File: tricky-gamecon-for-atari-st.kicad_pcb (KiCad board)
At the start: 2 copper layers, 14 parts, among them J1 Conn_01x09, SW1 GrayHill_series_78_SPDT_DIP_x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, SW2 SW_SPST, SW3 SW_SPST, SW4 SW_SPST, SW5 SW_SPST, SW6 SW_SPST, SW7 SW_SPST, SW8 SW_SPST, SW9 SW_SPST

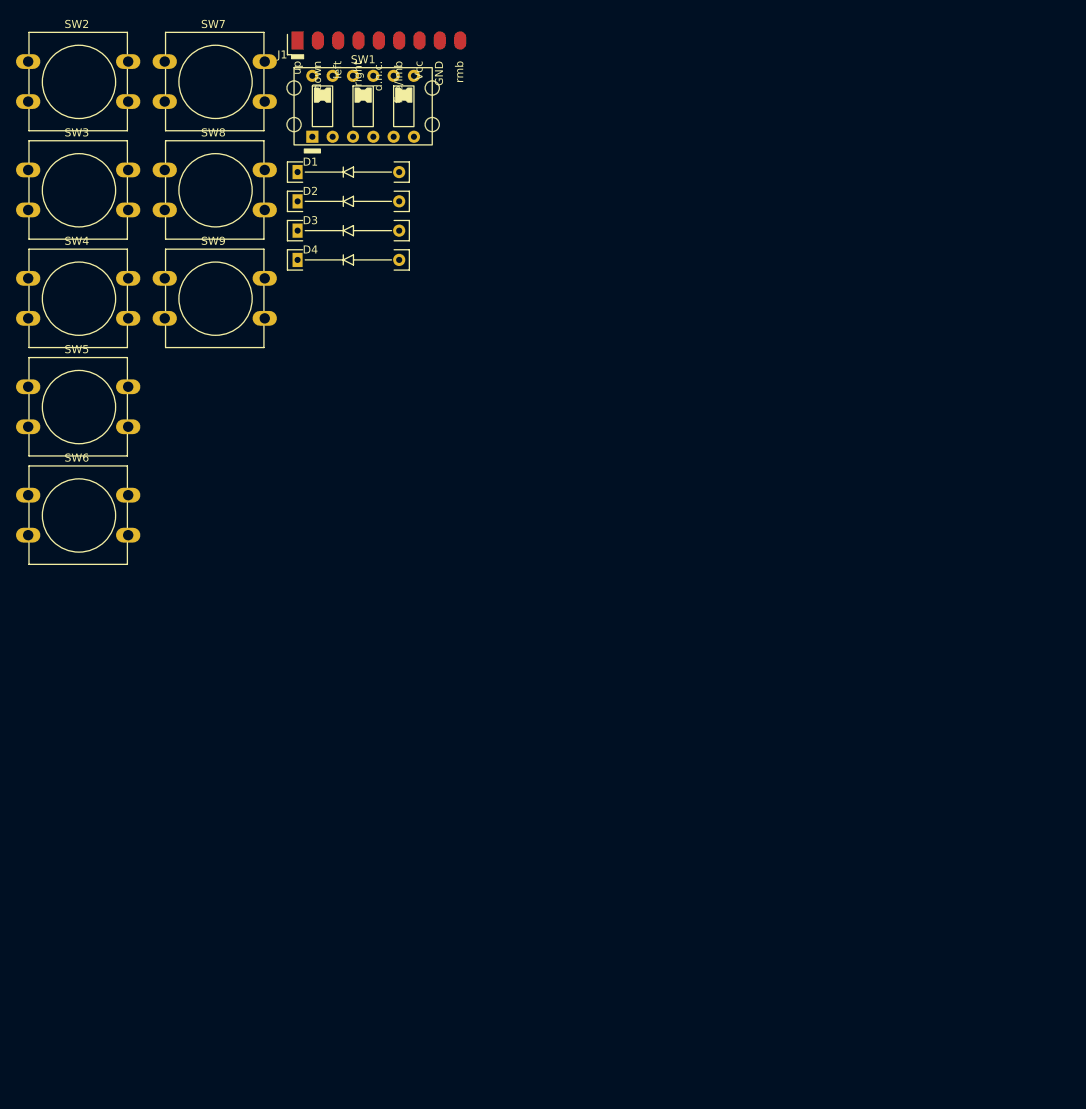
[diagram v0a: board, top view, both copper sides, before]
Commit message: initial tracing
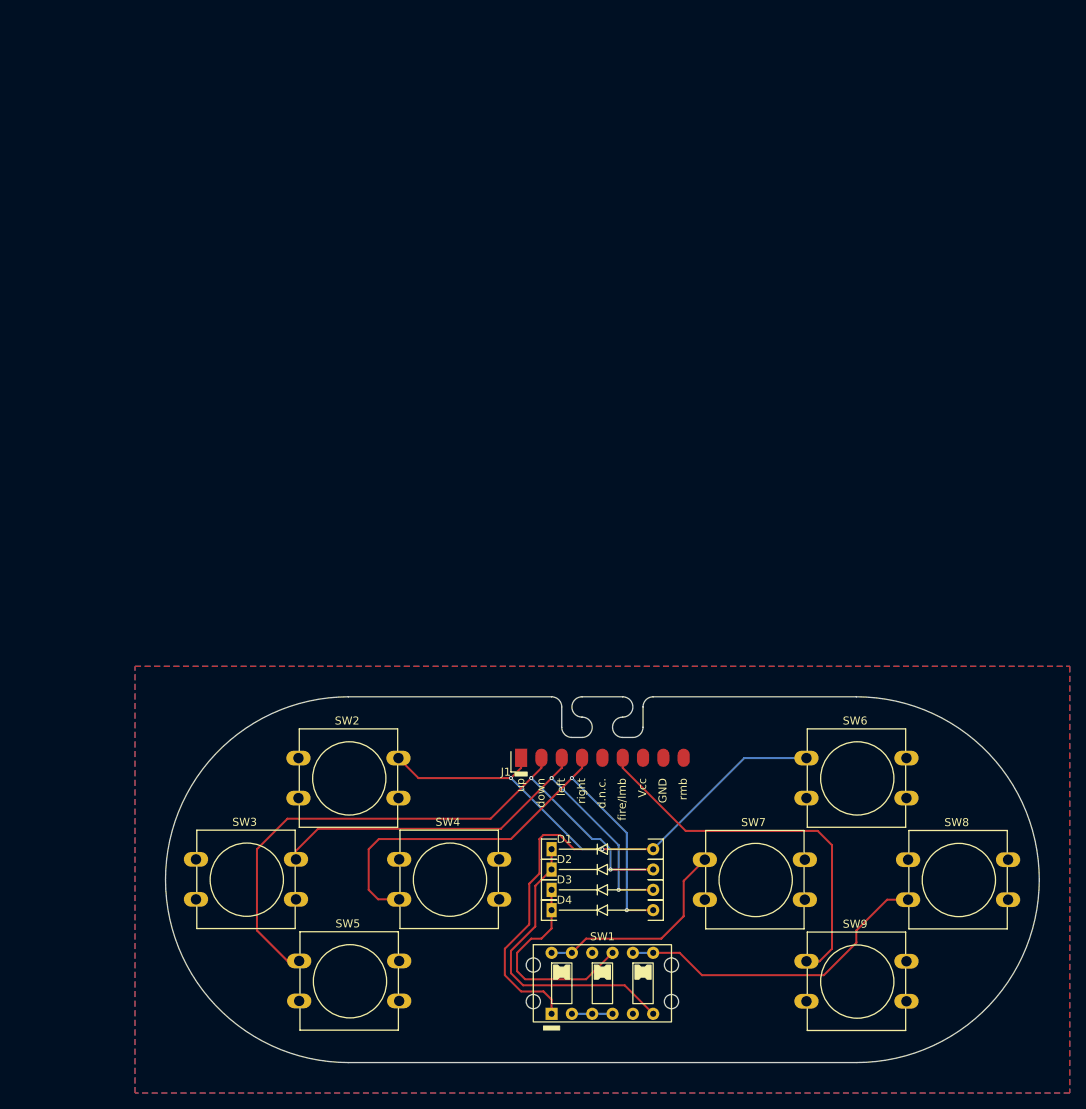
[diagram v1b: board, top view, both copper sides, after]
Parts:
- moved SW8 126.8 mm to (127.1, 118.2)
- moved SW7 120.5 mm to (101.7, 118.2)
- moved SW9 117.1 mm to (114.4, 130.8)
- moved SW1 113.6 mm to (88.9, 133.6)
- moved SW6 102.7 mm to (114.4, 105.5)
- moved J1 93.9 mm to (88.9, 105.4)
- moved SW2 93.4 mm to (50.9, 105.5)
- moved D1 90.4 mm to (88.9, 116.8)
- moved D2 89.4 mm to (88.9, 119.4)
- moved SW3 88.7 mm to (38.1, 118.1)
- moved D3 88.3 mm to (88.9, 121.9)
- moved D4 87.3 mm to (88.9, 124.5)
- moved SW4 86.2 mm to (63.5, 118.1)
- moved SW5 79.4 mm to (51.0, 130.8)
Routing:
- net /up: track 0.00 -> 100.0 mm, vias 0 -> 2
- net /down: track 0.00 -> 79.5 mm, vias 0 -> 2
- net /right: track 0.00 -> 64.2 mm, vias 0 -> 2
- net /left: track 0.00 -> 61.6 mm, vias 0 -> 2
- net /fire/lmb: track 0.00 -> 48.2 mm
- net /special_1: track 0.00 -> 40.4 mm
- net Net-(D1-K): track 0.00 -> 37.5 mm
- net /special_2: track 0.00 -> 26.6 mm
- net Net-(D3-K): track 0.00 -> 26.4 mm
- net Net-(SW1-Pad2): track 0.00 -> 5.08 mm
- added copper zone on B.Cu, net GND
- added copper zone on F.Cu, net GND
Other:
- board outline added: 109.2 x 45.7 mm
